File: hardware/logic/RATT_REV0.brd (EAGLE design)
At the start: 127 x 76.2 mm, 126 parts, among them IC1 TLP292-4, IC13 MCP73832, IC16 PCA9539PW, IC2 CPC1002N, IC200 TPS2115AIPWRQ1, IC3 CPC1002N, IC300 MAX98357, IC4 CPC1002N, IC5 CPC1002N, IC500 AP2112K-3.3V, J1 4P-2.0, J2 4P-2.0, J4 4P-2.0, J5 F-1X04-SIP-100-40, J6 4P-2.0, J7 PHOENIX1803484, J8 PHOENIX1803484, Q5 2N7002, U1 RPI-ZERO

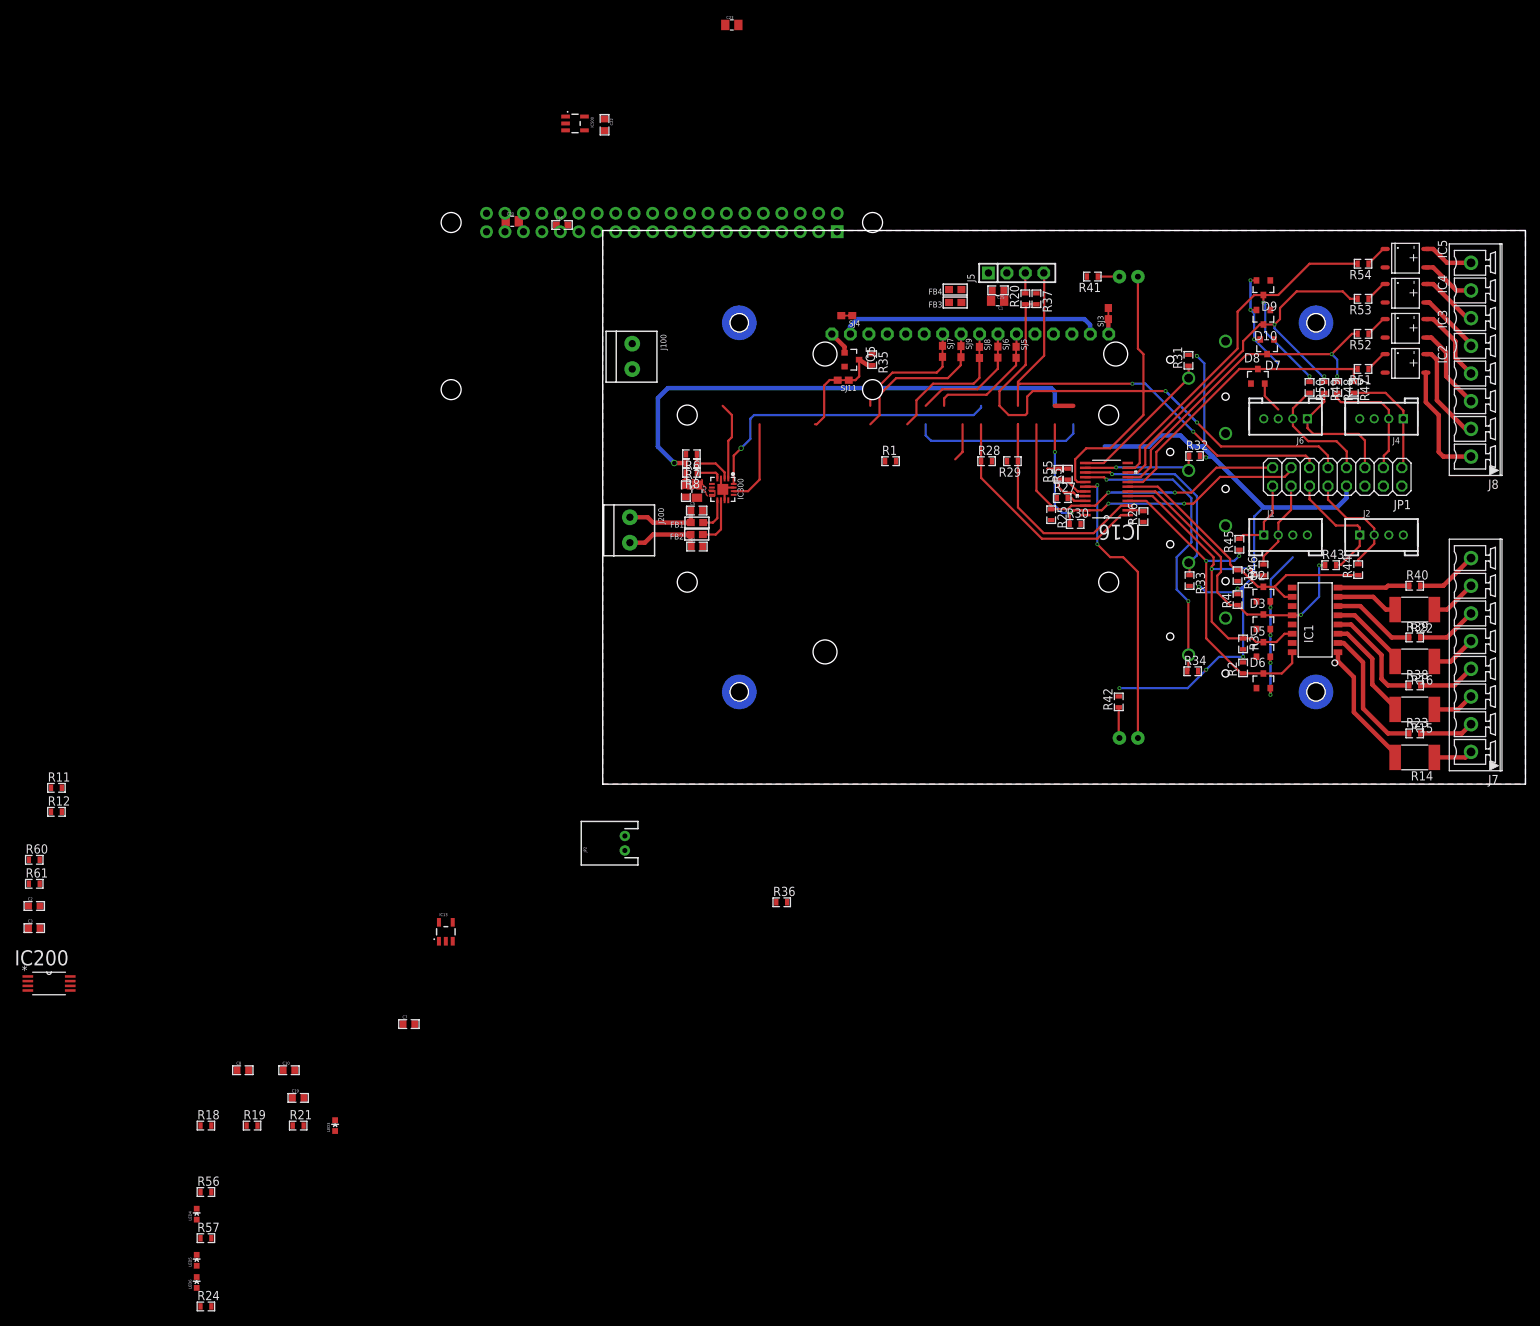
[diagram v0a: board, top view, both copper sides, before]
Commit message: most stuff placed
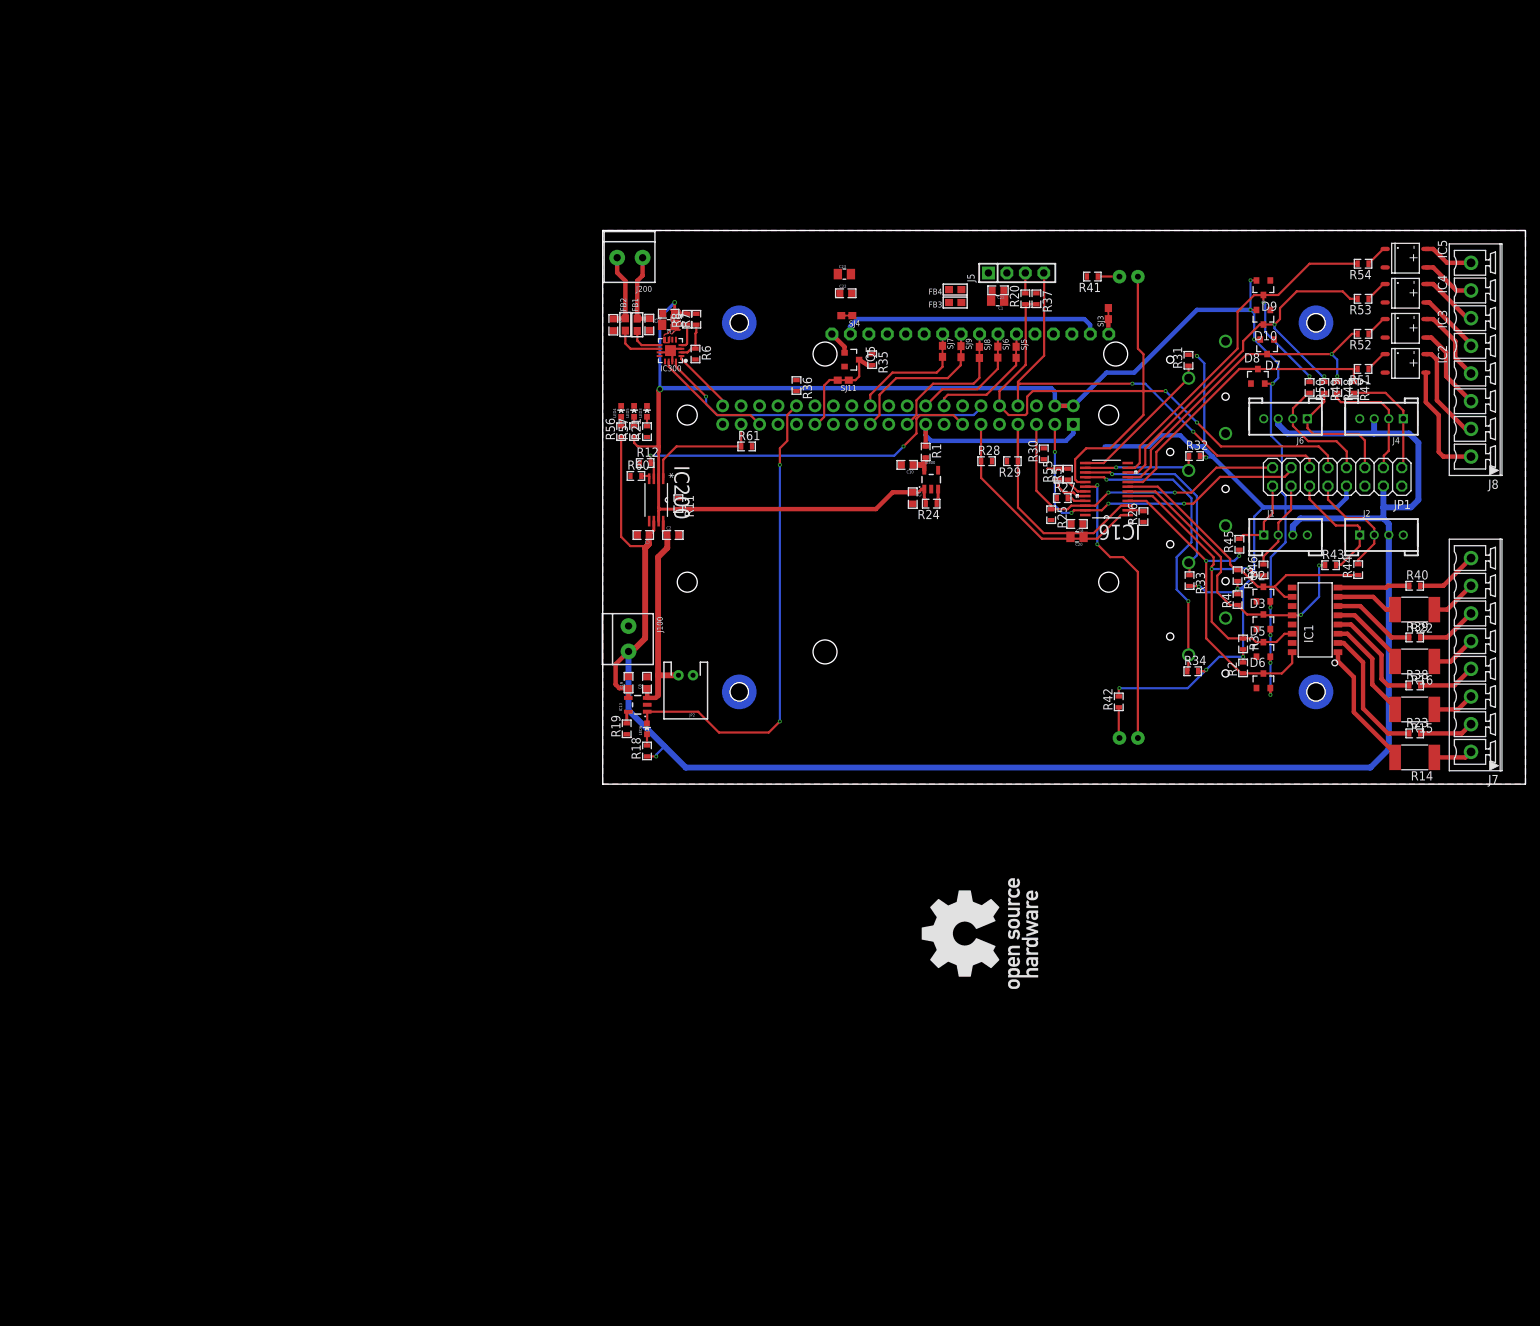
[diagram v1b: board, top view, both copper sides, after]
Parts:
- moved R24 148.9 mm to (45.2, 38.6), turned to 180 degrees
- moved LED5 131.4 mm to (4.32, 51.3)
- moved R57 125.7 mm to (4.32, 48.5), turned to 90 degrees
- moved LED4 125.0 mm to (2.54, 51.3)
- moved R56 119.2 mm to (2.54, 48.5), turned to 90 degrees
- moved C10 119.1 mm to (41.9, 43.9), turned to 180 degrees
- moved R61 115.0 mm to (19.8, 46.5)
- moved LED3 107.3 mm to (6.10, 51.3)
- moved R21 106.9 mm to (6.10, 48.5), turned to 90 degrees
- moved IC200 106.8 mm to (7.37, 39.1), turned to 270 degrees
- moved C2 101.6 mm to (9.65, 34.3)
- moved C7 100.2 mm to (42.7, 39.4), turned to 270 degrees
- moved C3 99.8 mm to (5.59, 34.3), turned to 180 degrees
- moved R60 98.2 mm to (4.57, 42.4)
- moved LED6 98.2 mm to (6.10, 7.62)
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- renumbered U1 to J87
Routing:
- net +5VIN: track 0.00 -> 253.2 mm, vias 0 -> 1
- net +5VB: track 116.6 -> 237.8 mm, vias 8 -> 10
- net CHARGE_STATUS: track 0.00 -> 66.1 mm, vias 0 -> 2
- net SHUTDOWN: track 5.25 -> 50.5 mm, vias 0 -> 2
- net V_BATT: track 0.00 -> 30.5 mm
- net !PWR_LOSS: track 0.00 -> 17.2 mm
- net +3.3V: track 105.2 -> 116.1 mm
- net I2S_WS/LRCLK: track 11.8 -> 16.5 mm
- net I2S_BCK: track 42.6 -> 46.7 mm
- net 3V3: track 23.9 -> 26.9 mm
- net N$18: track 0.00 -> 2.08 mm
- net N$14: track 0.00 -> 1.69 mm
- net I2C_SDA: track 48.5 -> 46.9 mm
- net N$17: track 0.00 -> 1.55 mm
- net I2S_DOUT: track 10.7 -> 9.20 mm
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
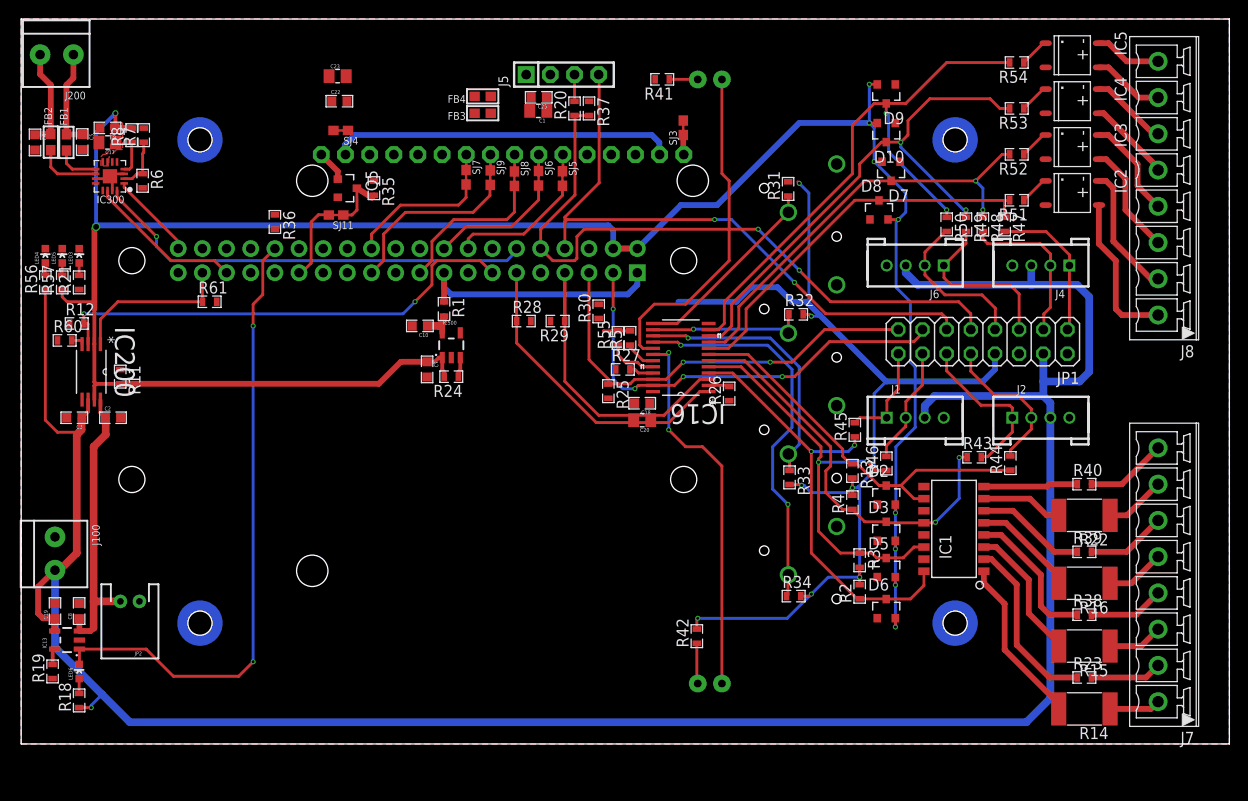
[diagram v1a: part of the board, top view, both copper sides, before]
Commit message: Added some stuff
Added clamps to RFID, added 1206 series resistor to LCD backlight
power in connector updated
lipo connector moved
played with cut away of plane
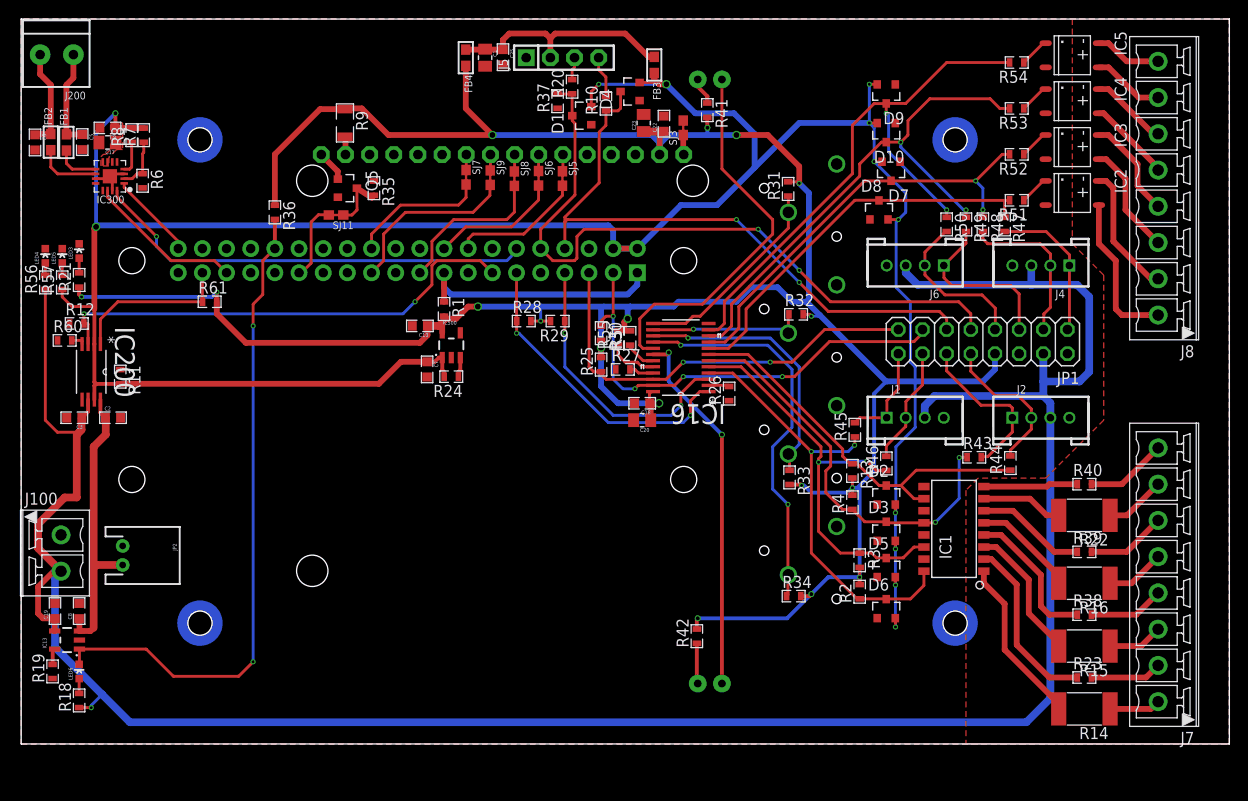
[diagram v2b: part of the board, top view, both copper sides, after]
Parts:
- removed SJ4: JUMPER-PAD-2-NC_BY_TRACE, MakeItLabs:SOLDERJUMPER_10MIL
- added D1, D4: BAT54S, MakeItLabs:SOT-23
- added R10: 100R, MakeItLabs:0603-RES
- added R9: 10R, MakeItLabs:1206-RES
- J100: value (none) -> PHOENIX1803426; device MakeItLabs:TERMBLOCK_1X2-3.5MM -> MakeItLabs:1803426
- moved C22 34.2 mm to (67.6, 65.2), turned to 90 degrees
- moved C23 32.5 mm to (65.4, 65.3), turned to 90 degrees
- moved FB3 18.7 mm to (66.5, 71.4), turned to 270 degrees
- moved C1 7.90 mm to (48.8, 72.1), turned to 270 degrees
- moved R41 5.74 mm to (72.1, 66.6), turned to 270 degrees
- moved C25 5.65 mm to (50.6, 72.2), turned to 270 degrees
- moved JP2 4.89 mm to (10.7, 19.8), turned to 270 degrees
- moved FB4 4.44 mm to (46.7, 72.1), turned to 270 degrees
- moved R37 3.39 mm to (56.4, 67.6), turned to 90 degrees
- moved R25 2.90 mm to (61.0, 39.9), turned to 90 degrees
- moved R30 2.30 mm to (61.0, 43.2), turned to 270 degrees
- moved R20 2.30 mm to (57.9, 69.1)
- moved J5 1.78 mm to (56.9, 72.1)
- moved R36 1.02 mm to (26.7, 55.9)
- moved LED3 0.51 mm to (6.10, 51.8)
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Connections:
- removed net N$26: LCD3.15, LCD3.2, SJ4.1
- new net N$10: J5.4, R10.2
- new net N$9: LCD3.15, R9.2
- net +3.3V: now also LCD3.2, R9.1; no longer SJ4.2
- net +5VB: now also D1.2, D4.2
- net +5VIN: now also J100.2; no longer J100.1
- net GND: now also D1.1, D4.1, J100.1; no longer J100.2
- net RFID_RX: now also D4.3, R10.1; no longer J5.4
- net RFID_TX: now also D1.3
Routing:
- net +3.3V: track 116.1 -> 296.3 mm, vias 7 -> 17
- net N$26: track 36.2 -> 0.00 mm
- net +5VB: track 237.8 -> 269.6 mm, vias 10 -> 12
- net N$51: track 0.00 -> 24.6 mm
- net !I/O_RESET: track 34.7 -> 29.4 mm, vias 0 -> 2
- net LED0: track 35.6 -> 40.4 mm
- net N$10: track 0.00 -> 4.39 mm
- net +5VIN: track 253.2 -> 256.3 mm
- net CHARGE_STATUS: track 66.1 -> 69.1 mm
- net RFID_TX: track 70.8 -> 73.2 mm
- net I2C_SDA: track 46.9 -> 48.9 mm
- net N$9: track 0.00 -> 1.90 mm
- net LED1: track 39.9 -> 38.8 mm
- net !BUTTON0: track 20.8 -> 21.8 mm
- net !I/O_IRQ: track 32.4 -> 32.7 mm, vias 0 -> 2
- added copper zone on layer 1, net +5VB
- added copper zone on layer 1, net N$16
- removed copper zone on layer 1, net VIN
